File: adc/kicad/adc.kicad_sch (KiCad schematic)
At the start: 106 parts, among them J1 Conn_01x02_Pin, J2 Conn_01x02_Pin, J3 Conn_01x02_Pin, J5 Conn_01x07_Pin, J6 pcie_98, U1 ADS1261B, U2 ESD5344D-TP, U3 TPS7A2050PDBVR, U4 TPS7A2025PDBVR, U6 TPS65135, U7 ADP7182AUJZ-5.0, U8 ADP7182AUJZ-2.5, U9 XC6206P332MR

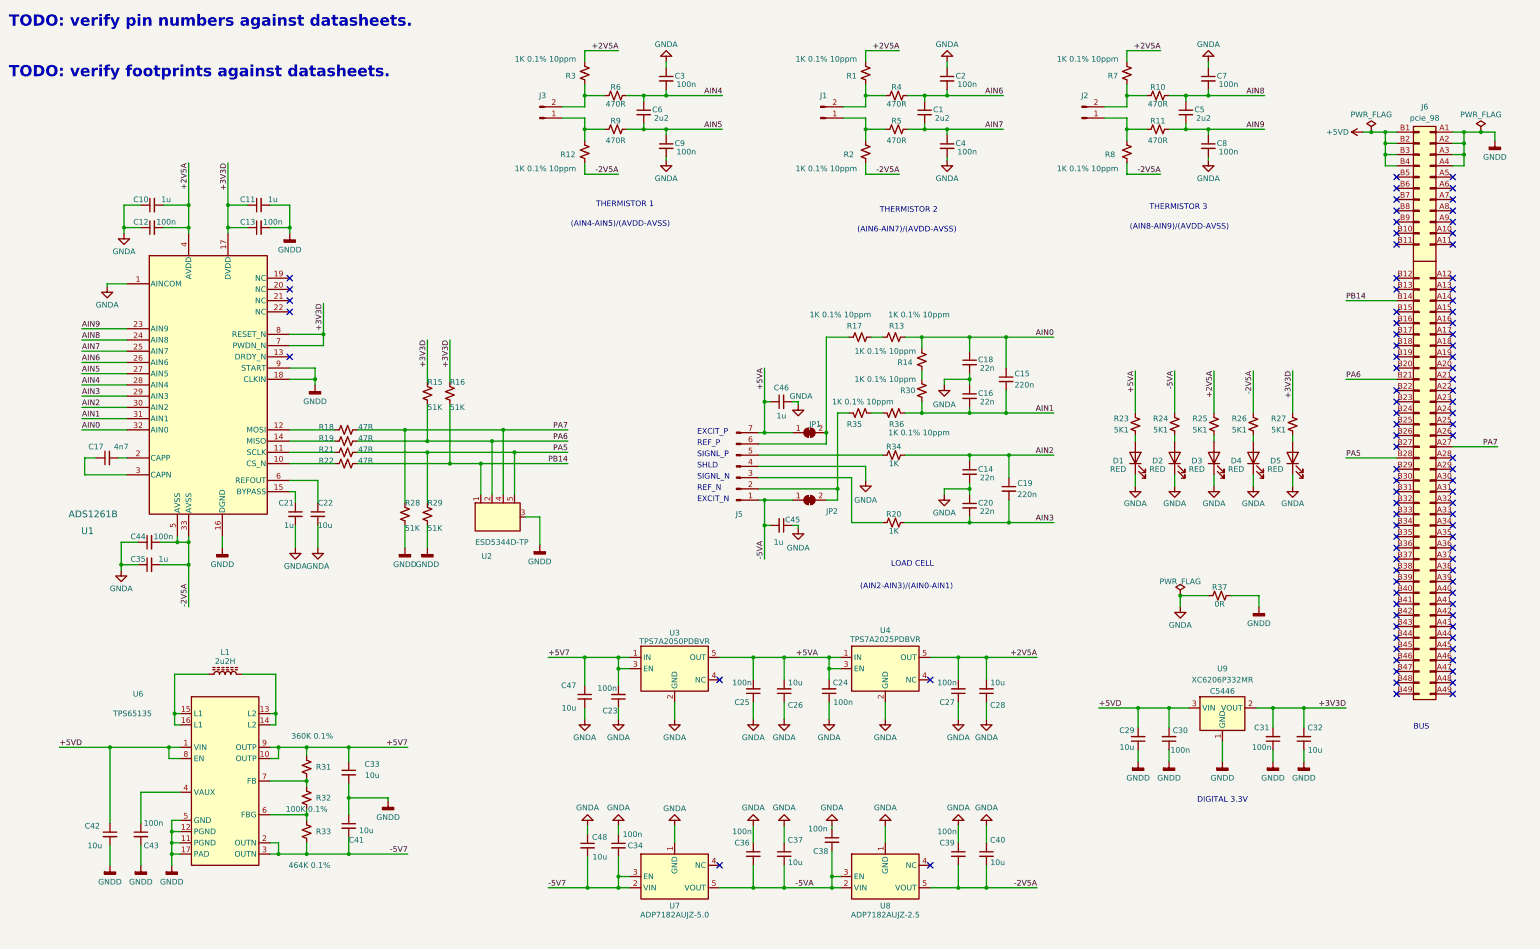
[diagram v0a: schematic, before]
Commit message: ADC layout is feature complete.
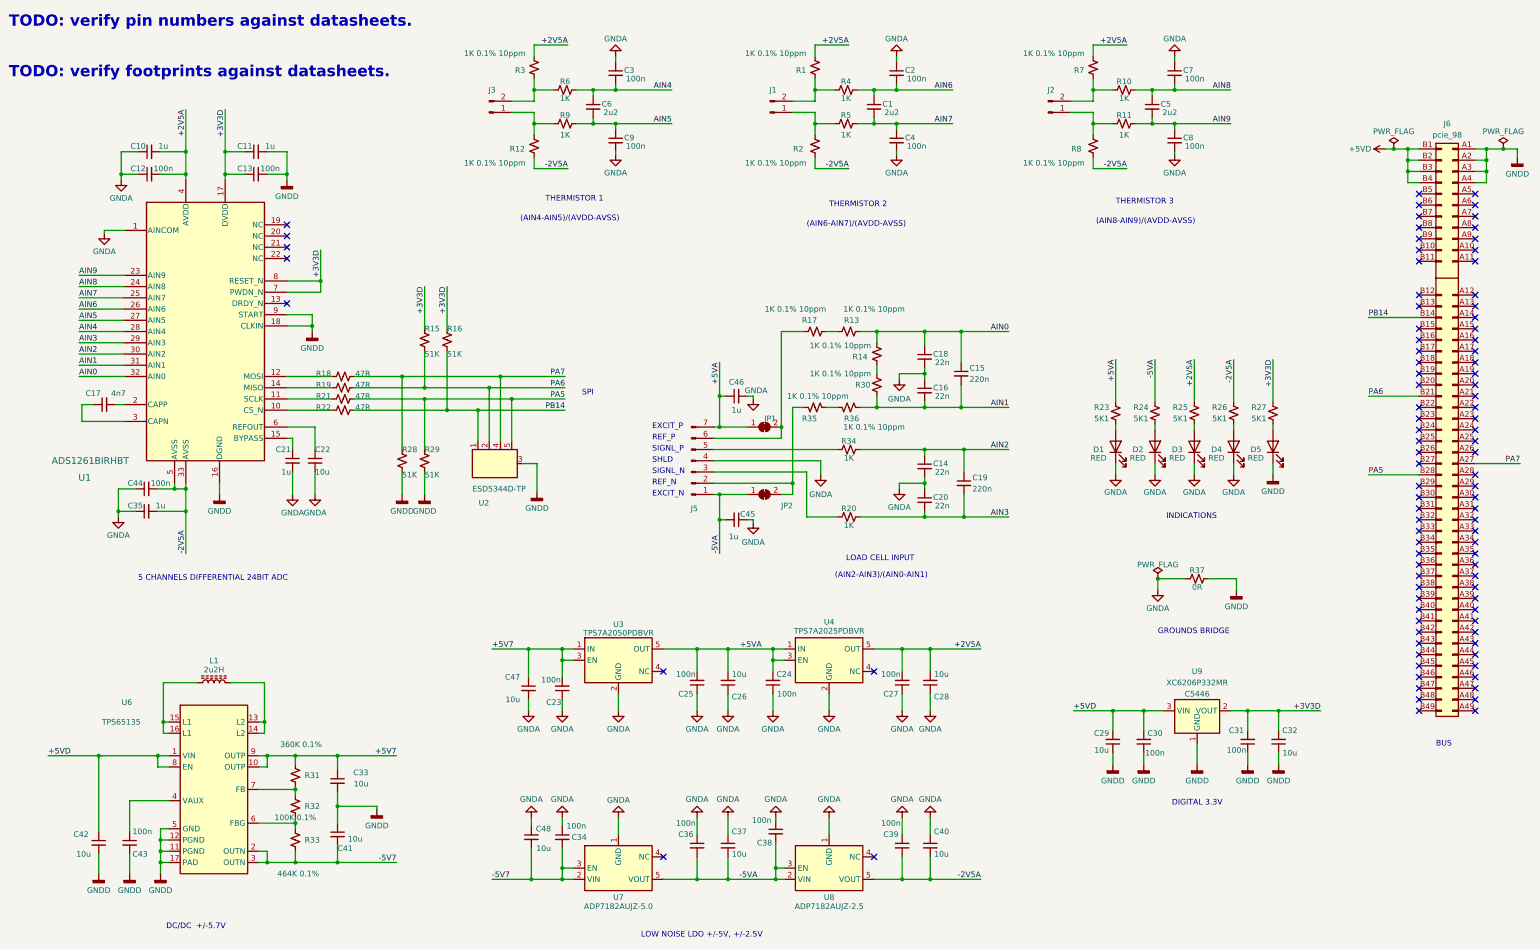
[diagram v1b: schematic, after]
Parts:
- J1, J2, J3: LCSC DNP -> C30436
- J5: LCSC DNP -> C70896
- J6, JP1, JP2: now left out of the parts list
- R10, R11, R4, R5, R6, R9: value 470R -> 1K; LCSC C25117 -> C11702
- U1: value ADS1261B -> ADS1261BIRHBT; LCSC DIGIKEY -> C2669964
- U3: LCSC DIGIKEY -> C2864504
- U4: value TPS7A2025PDBVR -> TPS7A2025PDBVRr; LCSC DIGIKEY -> C2869949
- U7: LCSC DIGIKEY -> C514357
- U8: LCSC DIGIKEY -> C462196
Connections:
- net GNDA: no longer D5.1 (K)
- net GNDD: now also D5.1 (K)
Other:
- note added: "5 CHANNELS DIFFERENTIAL 24BIT ADC"
- note added: "DC/DC +/-5.7V"
- note added: "GROUNDS BRIDGE"
- note added: "INDICATIONS"
- note added: "LOAD CELL INPUT"
- note added: "LOW NOISE LDO +/-5V, +/-2.5V"
- note added: "SPI"
- note removed: "LOAD CELL"
- title: ADS1261 ADC BOARD -> ADS1261B ADC BOARD
- moved on the sheet: C1, C10, C11, C12, C13, C14, C15, C16, C17, C18, C19, C2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
